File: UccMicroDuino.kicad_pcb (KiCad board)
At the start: 2 copper layers, 45.5 x 45 mm, 14 parts, among them J1 Pcb USB type A, J2 Header, U1 ATtiny85-20S

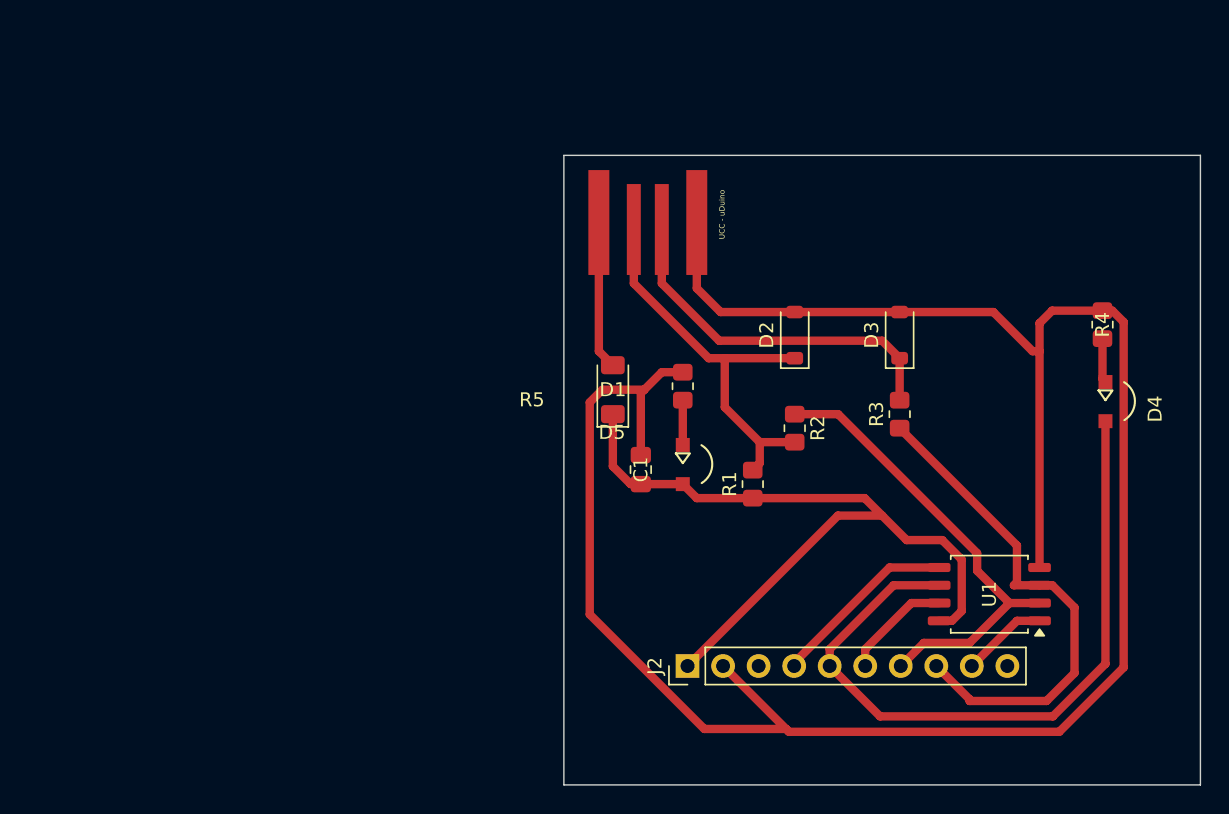
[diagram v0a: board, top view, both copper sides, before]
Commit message: Mi primer cambio para el practico 2
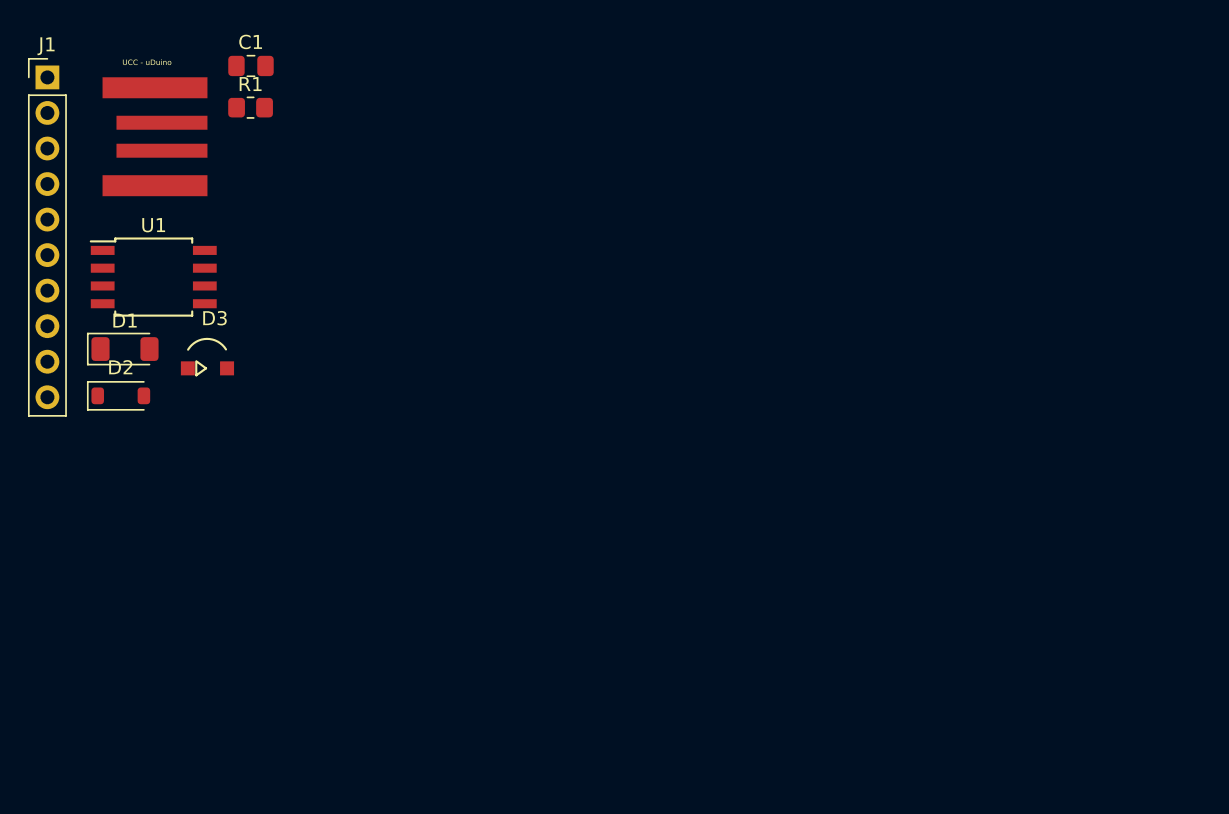
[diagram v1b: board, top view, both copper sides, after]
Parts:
- removed the D3 at (185.0, 86.3)
- removed D4: Led green, ledSmd:ledSMD
- removed R2, R3: 68Ω 5% 1/8W, Resistor_SMD:R_0805_2012Metric_Pad1.20x1.40mm_HandSolder
- removed R4, R5: 330Ω 5% 1/8W, Resistor_SMD:R_0805_2012Metric_Pad1.20x1.40mm_HandSolder
- D2: value 3.6V 1/2 mW -> D_Zener
- D3: renamed from D5; value LED RED -> LED
- J1: renamed from J2; value Header -> Conn_01x10_Socket
- J2: renamed from J1; value Pcb USB type A -> USB_A
- R1: value 1.5KΩ 5% 1/8W -> R
- U1: footprint Package_SO:SOIC-8_5.3x5.3mm_P1.27mm -> Package_SO:SOIC-8W_5.3x5.3mm_P1.27mm
- moved U1 63.9 mm to (131.7, 82.2), turned to 0 degrees
- moved J1 62.2 mm to (124.1, 67.9), turned to 0 degrees
- moved D2 48.4 mm to (129.3, 90.7), turned to 0 degrees
- moved R1 44.9 mm to (138.6, 70.1), turned to 0 degrees
- moved C1 40.1 mm to (138.6, 67.1), turned to 0 degrees
- moved J2 35.6 mm to (132.0, 72.2), turned to 0 degrees
- moved D1 35.0 mm to (129.6, 87.3), turned to 0 degrees
- moved D3 34.4 mm to (135.9, 88.7), turned to 0 degrees
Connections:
- C1 pad 1: +5V -> unconnected-(C1-Pad1)
- C1 pad 2: GND -> unconnected-(C1-Pad2)
- D1 pad 2: Net-(D1-A) -> unconnected-(D1-A-Pad2)
- D2 pad 1: Net-(D2-K) -> unconnected-(D2-K-Pad1)
- D2 pad 2: GND -> unconnected-(D2-A-Pad2)
- D3 pad 1: Net-(D5-K) -> unconnected-(D3-K-Pad1)
- D3 pad 2: +5V -> unconnected-(D3-A-Pad2)
- J1 pad 1: +5V -> unconnected-(J1-Pin_1-Pad1)
- J1 pad 2: GND -> unconnected-(J1-Pin_2-Pad2)
- J1 pad 4: Net-(J2-Pin_4) -> unconnected-(J1-Pin_4-Pad4)
- J1 pad 5: Net-(D4-A) -> unconnected-(J1-Pin_5-Pad5)
- J1 pad 6: Net-(J2-Pin_6) -> unconnected-(J1-Pin_6-Pad6)
- J1 pad 7: Net-(J2-Pin_7) -> unconnected-(J1-Pin_7-Pad7)
- J1 pad 8: Net-(J2-Pin_8) -> unconnected-(J1-Pin_8-Pad8)
- J1 pad 9: Net-(J2-Pin_9) -> unconnected-(J1-Pin_9-Pad9)
- J2 pad 1: Net-(D1-A) -> unconnected-(J2-VBUS-Pad1)
- J2 pad 2: Net-(D2-K) -> unconnected-(J2-D--Pad2)
- J2 pad 3: Net-(D3-K) -> unconnected-(J2-D+-Pad3)
- J2 pad 4: GND -> unconnected-(J2-GND-Pad4)
- R1 pad 2: Net-(D2-K) -> unconnected-(R1-Pad2)
- U1 pad 1: Net-(J2-Pin_9) -> unconnected-(U1-~{RESET}/PB5-Pad1)
- U1 pad 2: Net-(J2-Pin_7) -> unconnected-(U1-XTAL1/PB3-Pad2)
- U1 pad 3: Net-(J2-Pin_8) -> unconnected-(U1-XTAL2/PB4-Pad3)
- U1 pad 4: GND -> unconnected-(U1-GND-Pad4)
- U1 pad 5: Net-(J2-Pin_4) -> unconnected-(U1-AREF/PB0-Pad5)
- U1 pad 6: Net-(D4-A) -> unconnected-(U1-PB1-Pad6)
- U1 pad 7: Net-(J2-Pin_6) -> unconnected-(U1-PB2-Pad7)
- U1 pad 8: +5V -> unconnected-(U1-VCC-Pad8)
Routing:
- net GND: track 157.3 -> 0.00 mm
- net +5V: track 55.4 -> 0.00 mm
- net Net-(D4-A): track 51.0 -> 0.00 mm
- net Net-(J2-Pin_8): track 36.3 -> 0.00 mm
- net Net-(J2-Pin_7): track 33.5 -> 0.00 mm
- net Net-(D2-K): track 29.3 -> 0.00 mm
- net Net-(D3-K): track 26.1 -> 0.00 mm
- net Net-(J2-Pin_4): track 13.4 -> 0.00 mm
- net Net-(D1-A): track 10.6 -> 0.00 mm
- net Net-(J2-Pin_6): track 7.85 -> 0.00 mm
- net Net-(J2-Pin_9): track 6.18 -> 0.00 mm
- net Net-(D5-K): track 3.20 -> 0.00 mm
- net Net-(D4-K): track 3.19 -> 0.00 mm
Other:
- board outline removed
